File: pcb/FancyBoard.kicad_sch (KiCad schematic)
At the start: 171 parts, among them J1 Conn_01x02_Socket, SW1 SW_Push_45deg, SW10 SW_Push_45deg, SW11 SW_Push_45deg, SW12 SW_Push_45deg, SW13 SW_Push_45deg, SW14 SW_Push_45deg, SW15 SW_Push_45deg, SW16 SW_Push_45deg, SW17 SW_Push_45deg, SW18 SW_Push_45deg, SW19 SW_Push_45deg, SW2 SW_Push_45deg, SW20 SW_Push_45deg, SW21 SW_Push_45deg, SW22 SW_Push_45deg, SW23 SW_Push_45deg, SW24 SW_Push_45deg, SW25 SW_Push_45deg, SW26 SW_Push_45deg, SW27 SW_Push_45deg, SW28 SW_Push_45deg, SW29 SW_Push_45deg, SW3 SW_Push_45deg, SW30 SW_Push_45deg, SW31 SW_Push_45deg, SW32 SW_Push_45deg, SW33 SW_Push_45deg, SW34 SW_Push_45deg, SW35 SW_Push_45deg, SW36 SW_Push_45deg, SW37 SW_Push_45deg, SW38 SW_Push_45deg, SW39 SW_Push_45deg, SW4 SW_Push_45deg, SW40 SW_Push_45deg, SW41 SW_Push_45deg, SW42 SW_Push_45deg, SW43 SW_Push_45deg, SW44 SW_Push_45deg, SW45 SW_Push_45deg, SW46 SW_Push_45deg, SW47 SW_Push_45deg, SW48 SW_Push_45deg, SW49 SW_Push_45deg, SW5 SW_Push_45deg, SW50 SW_Push_45deg, SW51 SW_Push_45deg, SW52 SW_Push_45deg, SW53 SW_Push_45deg, SW54 SW_Push_45deg, SW55 SW_Push_45deg, SW56 RotaryEncoder_Switch, SW57 RotaryEncoder_Switch, SW58 SW_SPDT, SW6 SW_Push_45deg, SW7 SW_Push_45deg, SW70 SW_Push_45deg, SW71 SW_Push_45deg, SW72 SW_Push_45deg, SW73 SW_Push_45deg, SW74 SW_Push_45deg, SW75 SW_Push_45deg, SW76 SW_Push_45deg, SW77 SW_Push_45deg, SW78 SW_Push_45deg, SW79 SW_Push_45deg, SW8 SW_Push_45deg, SW80 SW_Push_45deg, SW81 SW_Push_45deg, SW82 SW_Push_45deg, SW83 SW_Push_45deg, SW84 SW_Push_45deg, SW85 SW_Push_45deg, SW86 SW_Push_45deg, SW87 SW_Push_45deg, SW88 SW_Push_45deg, SW89 SW_Push_45deg, SW9 SW_Push_45deg, SW90 SW_Push_45deg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

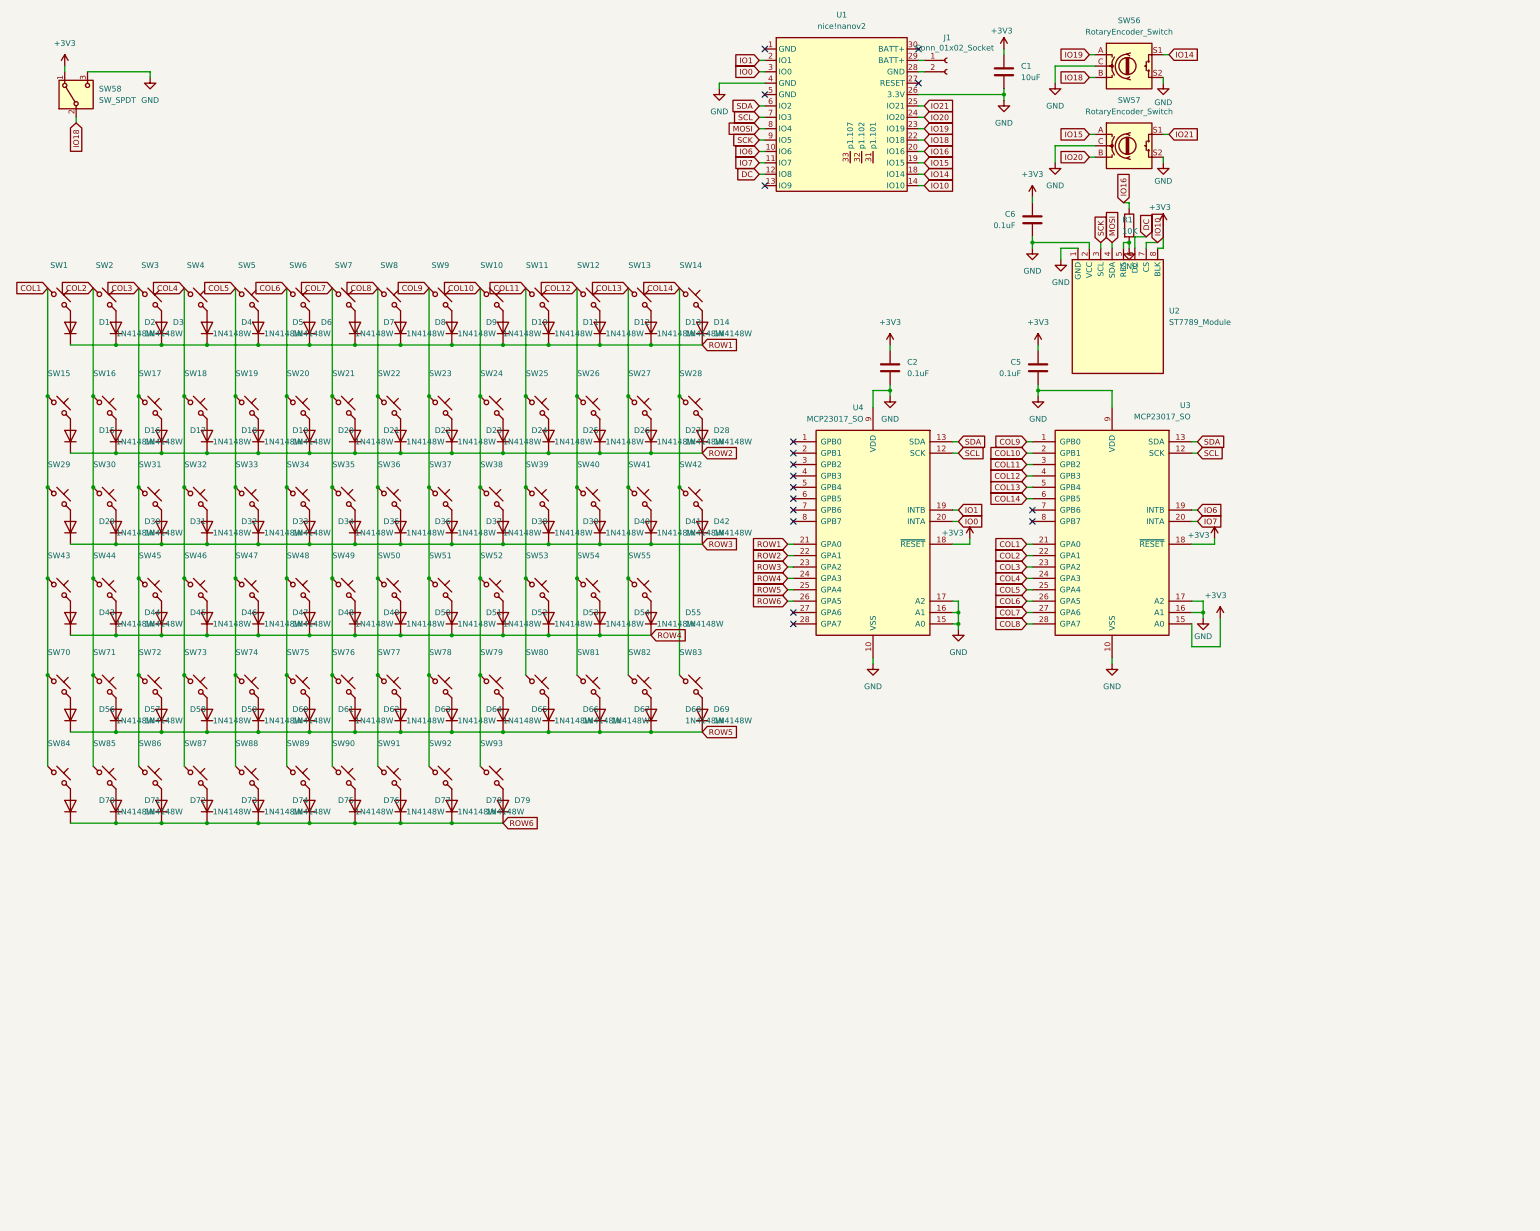
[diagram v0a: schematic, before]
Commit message: schematic done
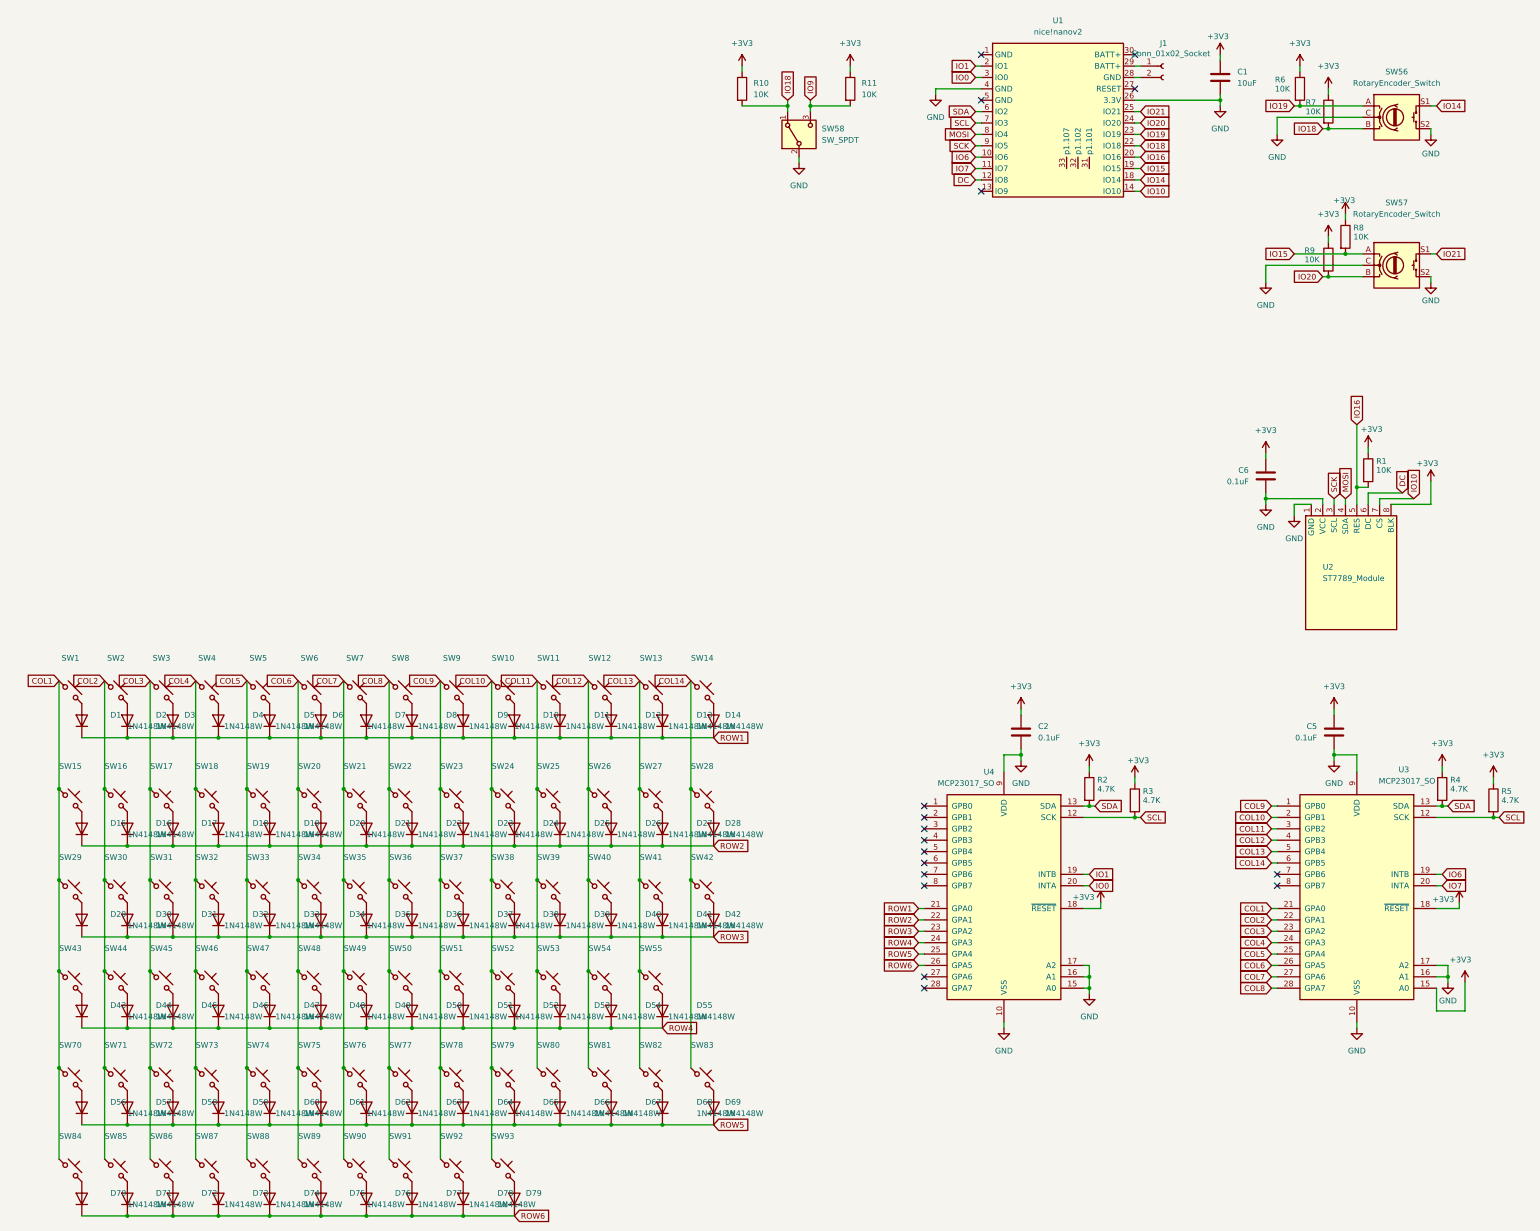
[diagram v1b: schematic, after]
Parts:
- added R10, R11, R6, R7, R8, R9: 10K, symbol Device:R
- added R2, R3, R4, R5: 4.7K, symbol Device:R
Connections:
- net +3V3: now also R1.1, R10.1, R11.1, R2.1, R3.1, R4.1, R5.1, R6.1, R7.1, R8.1, R9.1; no longer SW58.1 (A)
- net GND: now also SW58.2 (B); no longer R1.2, SW58.3 (C), U2.5 (RES)
- net IO15: now also R8.2
- net IO16: now also R1.2, U2.5 (RES); no longer R1.1
- net IO18: now also SW58.1 (A), R10.2, R7.2; no longer SW58.2 (B)
- net IO19: now also R6.2
- net IO20: now also R9.2
- net SCL: now also R3.2, R5.2
- net SDA: now also R2.2, R4.2
- new net IO9: R11.2, SW58.3 (C)
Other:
- moved on the sheet: C1, C2, C5, C6, D1, D10, D11, D12, D13, D14, D15, D16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
